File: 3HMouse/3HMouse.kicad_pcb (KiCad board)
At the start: 2 copper layers, 123.8 x 138.1 mm, 117 parts, among them J1 USB_C_Receptacle_USB2.0, SW0_0 CherryMX, SW0_1 CherryMX, SW0_2 CherryMX, SW1_0 CherryMX, SW1_1 CherryMX, SW1_2 CherryMX, SW2_0 CherryMX, SW2_1 CherryMX, SW2_2 CherryMX, SW3_0 CherryMX, SW3_1 CherryMX, SW3_2 CherryMX, SW3_3 CherryMX, SW3_4 CherryMX, SW4_0 CherryMX, SW4_1 CherryMX, SW4_2 CherryMX, SW4_3 CherryMX, SW4_4 CherryMX, SW5_0 CherryMX, SW5_1 CherryMX, SW5_2 CherryMX, SW5_3 CherryMX, SW5_4 CherryMX, SW6_0 CherryMX, SW6_1 CherryMX, SW6_2 CherryMX, SW6_3 CherryMX, SW6_4 CherryMX, U1 ATmega32U4-M, U2 USBLC6-2SC6, Y1 16 MHz

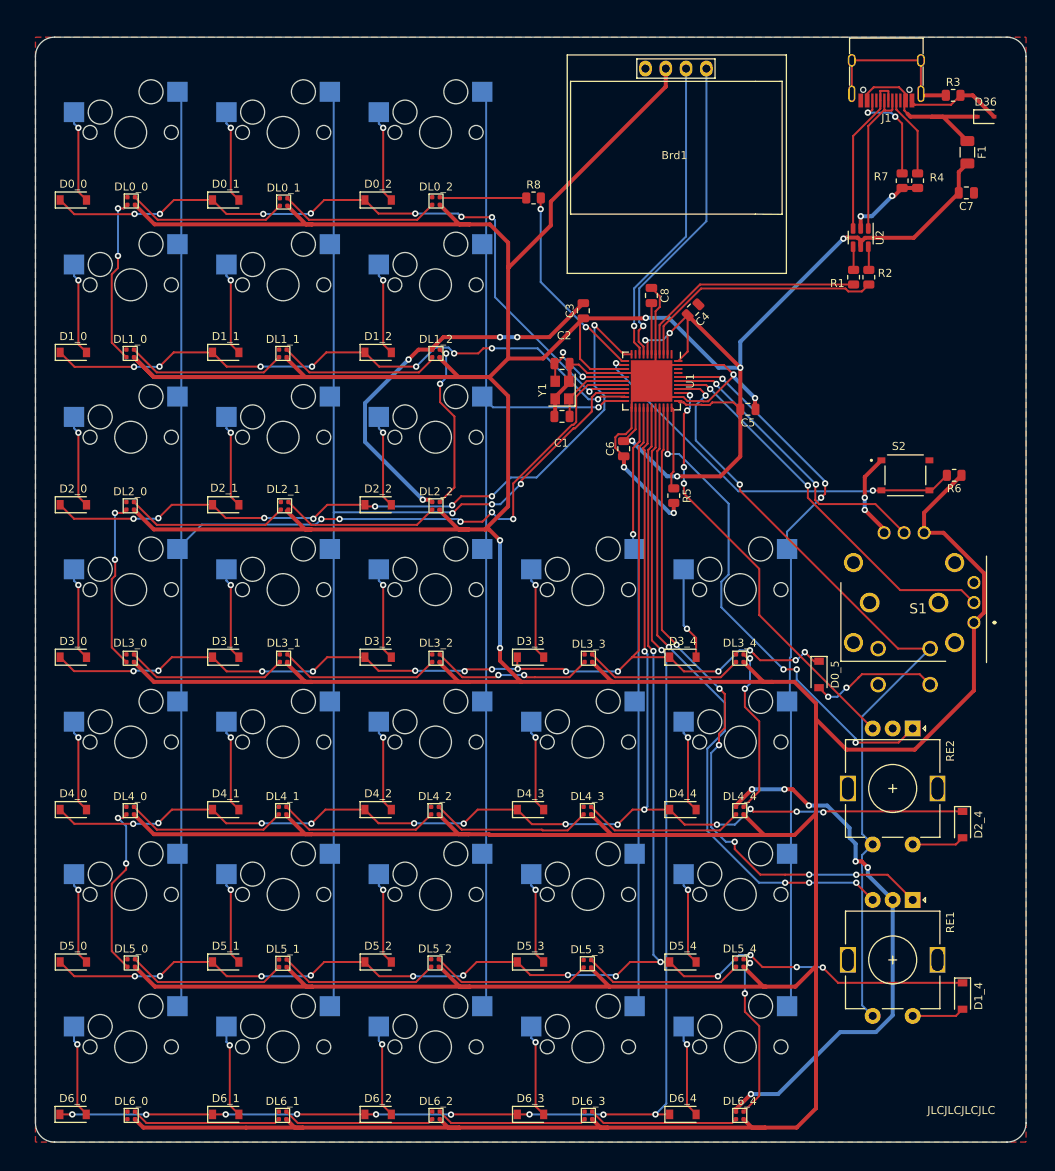
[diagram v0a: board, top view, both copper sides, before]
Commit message: v2.1.0
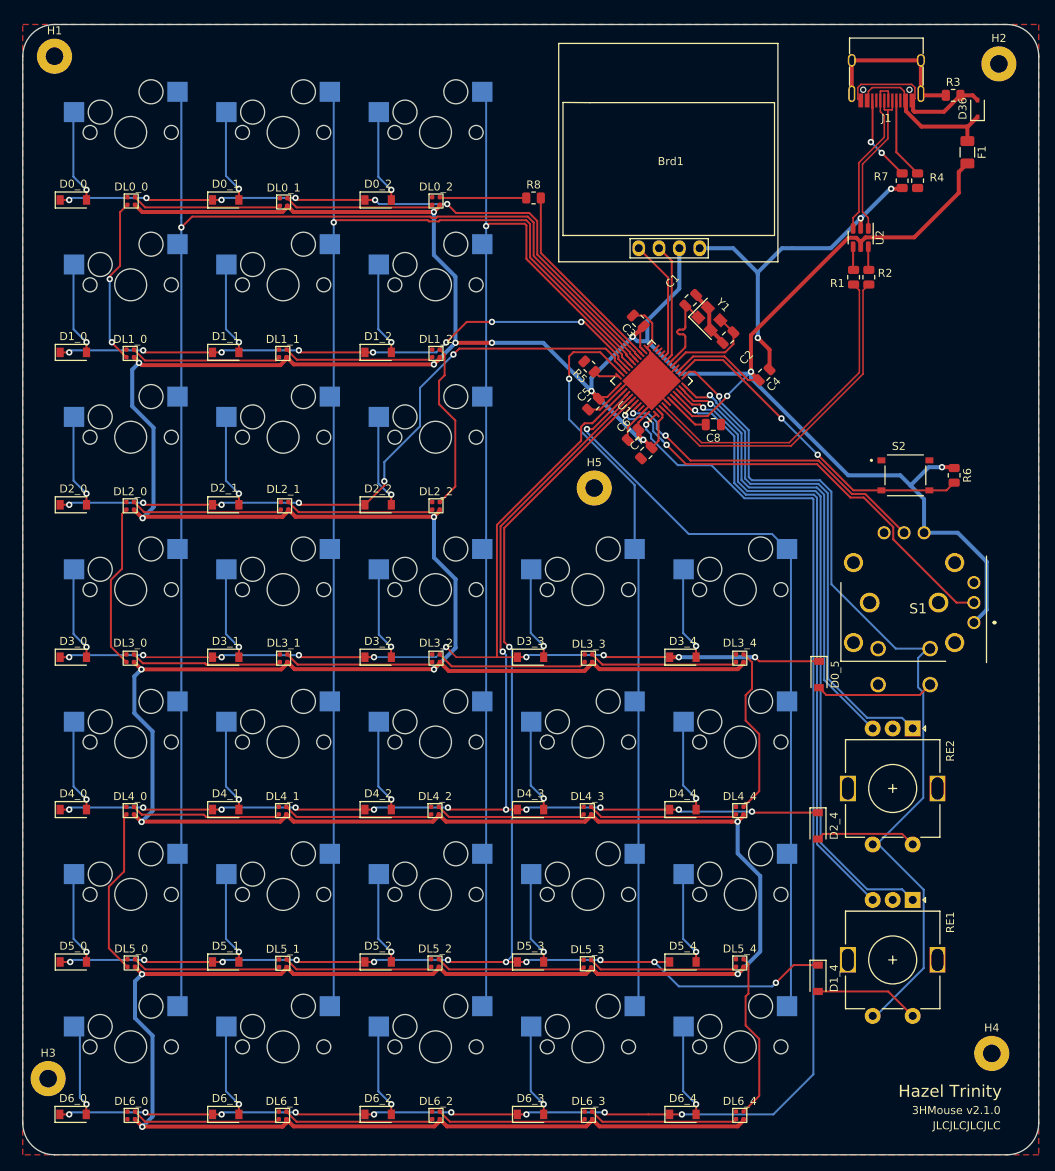
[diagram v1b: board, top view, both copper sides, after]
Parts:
- added H1: MountingHole, MountingHole:MountingHole_2.2mm_M2_Pad, F.Cu at (23.8, 23.8)
- added H2: MountingHole, MountingHole:MountingHole_2.2mm_M2_Pad, F.Cu at (141.9, 24.8)
- added H3: MountingHole, MountingHole:MountingHole_2.2mm_M2_Pad, F.Cu at (23.0, 151.6)
- added H4: MountingHole, MountingHole:MountingHole_2.2mm_M2_Pad, F.Cu at (141.0, 148.5)
- added H5: MountingHole, MountingHole:MountingHole_2.2mm_M2_Pad, F.Cu at (91.3, 77.8)
- moved C7 51.6 mm to (97.8, 73.4), turned to 45 degrees
- moved C1 21.7 mm to (103.3, 54.3), turned to 45 degrees
- moved C2 21.0 mm to (108.0, 59.0), turned to -135 degrees
- moved Y1 20.5 mm to (105.7, 56.6), turned to -45 degrees
- moved C5 19.3 mm to (91.2, 67.3), turned to 45 degrees
- moved R5 19.3 mm to (90.7, 62.6), turned to 135 degrees
- moved D1_4 18.2 mm to (119.3, 139.1)
- moved D2_4 18.1 mm to (119.3, 120.0)
- moved C8 17.9 mm to (106.2, 69.8), turned to 180 degrees
- moved C4 12.0 mm to (112.5, 63.6)
- moved C3 6.97 mm to (96.8, 56.9), turned to 135 degrees
- moved C6 2.11 mm to (96.1, 71.1), turned to 45 degrees
- moved D36 1.44 mm to (139.2, 30.4), turned to 90 degrees
- moved Brd1 1.34 mm to (100.8, 37.2), turned to 180 degrees
- turned R6 to -90 degrees
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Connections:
- net /D+F renamed /DF+
- net /D-F renamed /DF-
- net D+ I renamed DI+
- net D- I renamed DI-
- U1 pad 1: unconnected-(U1-Pad1) -> ROW6
- U1 pad 10: unconnected-(U1-Pad10) -> RE2B
- U1 pad 11: ROW2 -> RE2A
- U1 pad 12: LED -> COL5
- U1 pad 18: COL0 -> SCL
- U1 pad 19: ROW0 -> SDA
- U1 pad 20: COL1 -> unconnected-(U1-Pad20)
- U1 pad 21: ROW1 -> unconnected-(U1-Pad21)
- U1 pad 22: COL2 -> unconnected-(U1-Pad22)
- U1 pad 25: COL3 -> LED
- U1 pad 26: ROW3 -> ROW0
- U1 pad 27: ROW4 -> COL0
- U1 pad 28: ROW5 -> COL1
- U1 pad 29: ROW6 -> COL2
- U1 pad 30: RE1B -> ROW1
- U1 pad 31: RE1A -> ROW2
- U1 pad 32: RE2A -> COL3
- U1 pad 36: RE2B -> ROW3
- U1 pad 37: COL5 -> COL4
- U1 pad 38: VER -> ROW4
- U1 pad 39: HOR -> ROW5
- U1 pad 40: COL4 -> VER
- U1 pad 41: unconnected-(U1-Pad41) -> HOR
- U1 pad 8: SDA -> RE1B
- U1 pad 9: SCL -> RE1A
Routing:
- net +5V: track 981.9 -> 780.0 mm, vias 9 -> 20
- net GND: track 234.1 -> 109.8 mm, vias 18 -> 3
- net ROW6: track 166.2 -> 194.8 mm
- net SDA: track 39.9 -> 15.2 mm, vias 1 -> 0
- net SCL: track 38.7 -> 14.8 mm, vias 1 -> 0
- net ROW4: track 171.4 -> 153.2 mm, vias 14 -> 12
- net COL3: track 76.4 -> 93.7 mm
- net ROW5: track 192.1 -> 176.1 mm, vias 14 -> 12
- net /DF+: track 30.0 -> 41.2 mm
- net /DF-: track 31.6 -> 42.3 mm
- net COL5: track 101.5 -> 111.6 mm, vias 2 -> 1
- net COL2: track 135.4 -> 144.8 mm
- net ROW2: track 93.2 -> 84.2 mm, vias 8 -> 6
- net /RESET: track 50.4 -> 41.9 mm
- net VER: track 49.1 -> 57.1 mm
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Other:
- board size 123.8 x 138.1 mm -> 127 x 141.3 mm
- board text added: "3HMouse v2.1.0"
- board text added: "Hazel Trinity"

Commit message: v2.1.1
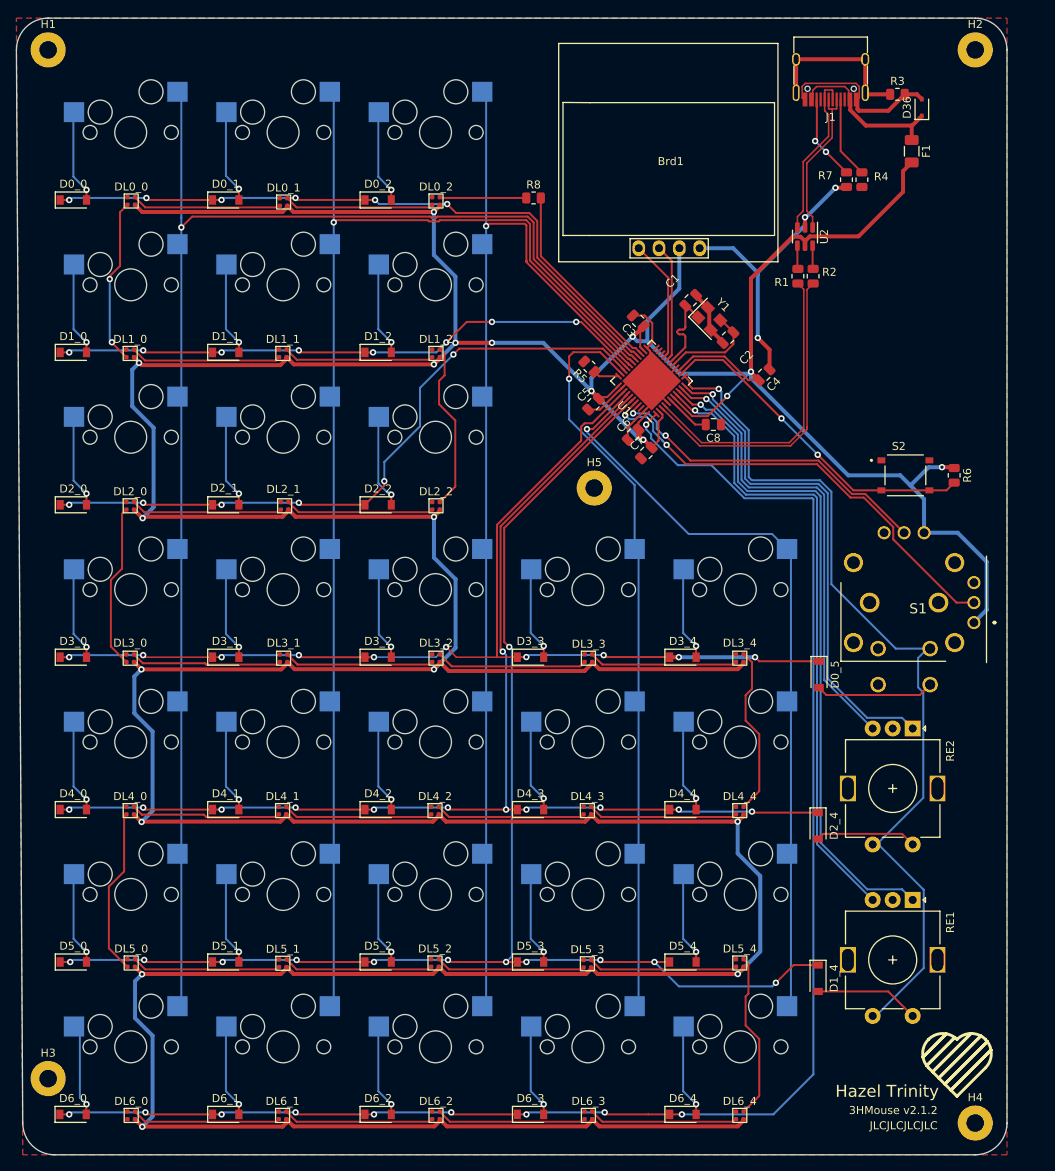
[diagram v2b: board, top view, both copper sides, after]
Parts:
- moved H4 8.94 mm to (138.9, 157.2)
- moved R4 6.96 mm to (124.7, 39.2)
- moved D36 6.96 mm to (132.2, 30.2)
- moved F1 6.96 mm to (131.0, 35.7)
- moved J1 6.96 mm to (120.8, 26.1)
- moved R2 6.96 mm to (118.6, 51.3)
- moved R3 6.96 mm to (129.2, 28.6)
- moved R7 6.96 mm to (122.8, 39.2)
- moved U2 6.96 mm to (117.6, 46.4)
- moved R1 6.96 mm to (116.7, 51.3)
- moved H2 3.43 mm to (138.9, 23.0)
- moved H1 1.12 mm to (23.0, 23.0)
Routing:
- net GND: track 109.8 -> 103.6 mm
- net /DF-: track 42.3 -> 39.5 mm
- net +5V: track 780.0 -> 777.2 mm
- net /DF+: track 41.2 -> 38.5 mm
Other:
- board size 127 x 141.3 mm -> 123.8 x 142.1 mm
- board text added: "3HMouse v2.1.2"
- board text removed: "3HMouse v2.1.0"
